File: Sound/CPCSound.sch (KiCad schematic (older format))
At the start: 8 parts, among them J903 Conn_01x08_Female

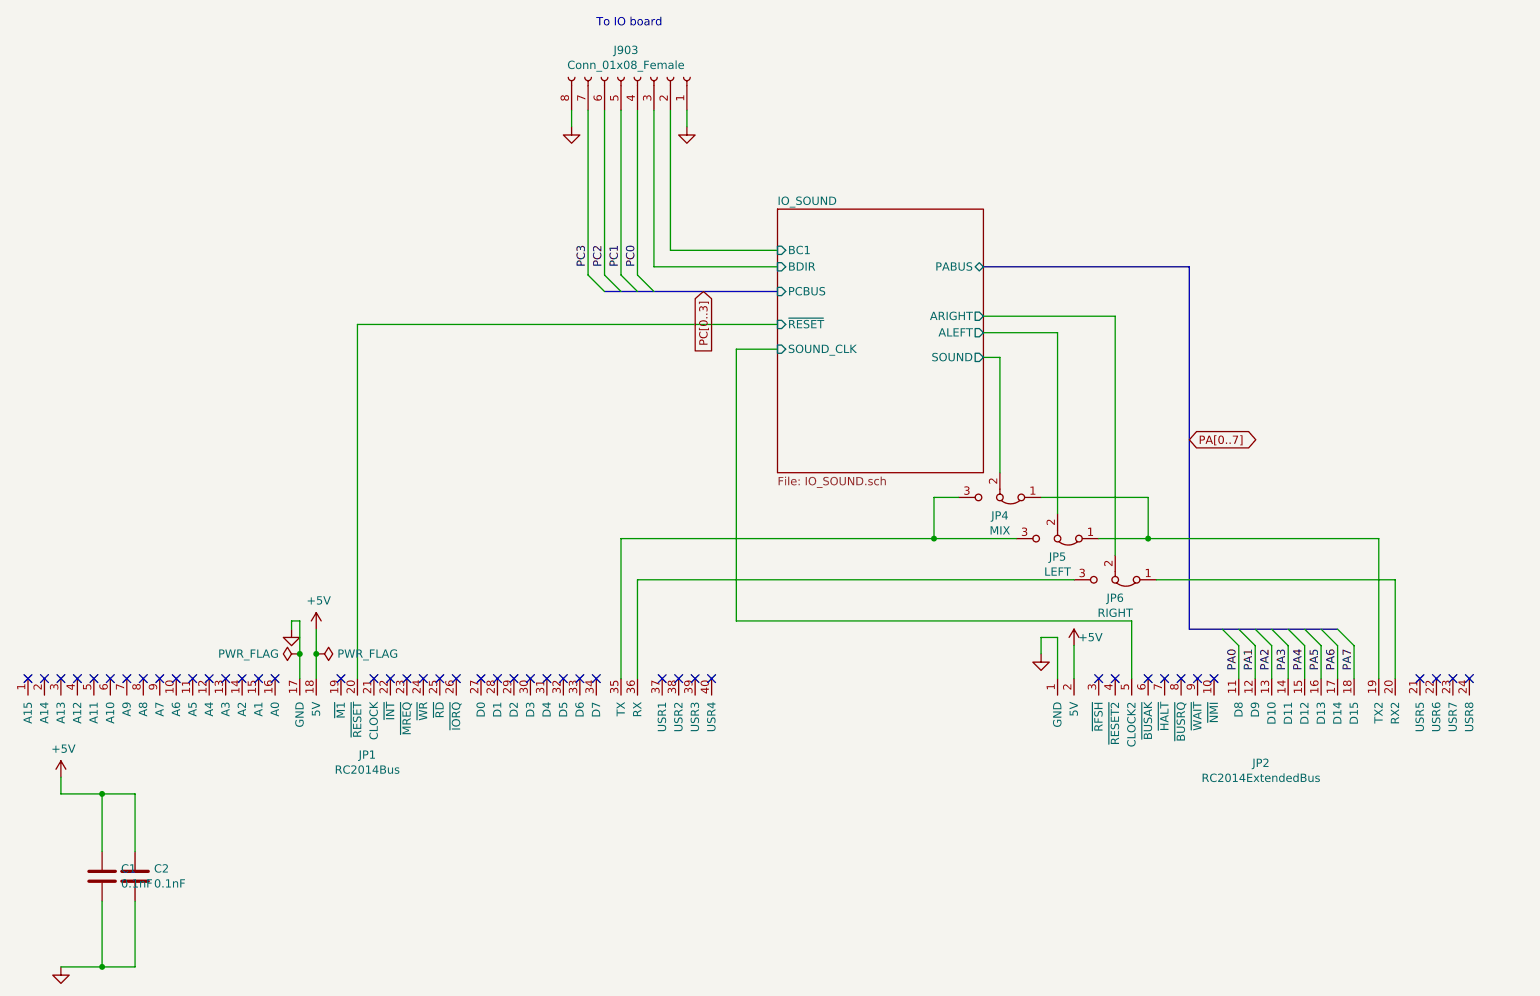
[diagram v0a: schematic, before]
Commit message: Long overdue update...
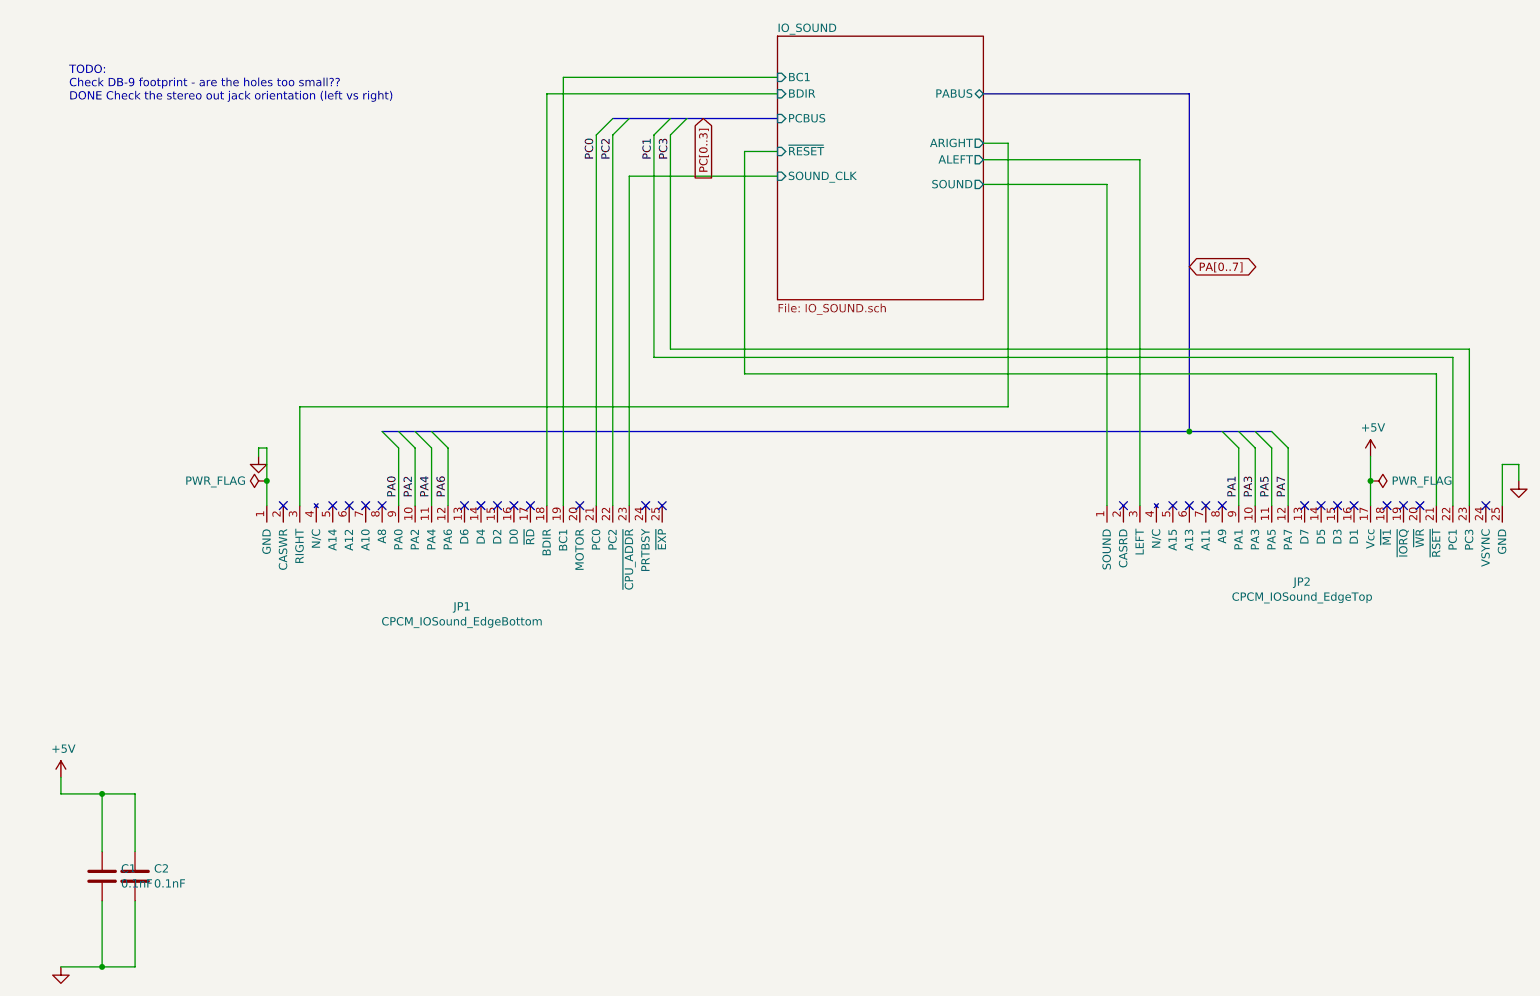
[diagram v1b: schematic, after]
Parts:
- removed J903: Conn_01x08_Female, Connector_PinSocket_2.54mm:PinSocket_1x08_P2.54mm_Vertical, symbol Connector:Conn_01x08_Female
- removed JP1: RC2014Bus, Connector_PinHeader_2.54mm:PinHeader_1x40_P2.54mm_Vertical, symbol CPCSound-rescue:RC2014Bus-CPC
- removed JP2: RC2014ExtendedBus, Connector_PinHeader_2.54mm:PinHeader_1x25_P2.54mm_Vertical, symbol CPCSound-rescue:RC2014ExtendedBus-CPC
- removed JP4: MIX, Connector_PinHeader_2.54mm:PinHeader_1x03_P2.54mm_Vertical, symbol Jumper:Jumper_3_Bridged12
- removed JP5: LEFT, Connector_PinHeader_2.54mm:PinHeader_1x03_P2.54mm_Vertical, symbol Jumper:Jumper_3_Bridged12
- removed JP6: RIGHT, Connector_PinHeader_2.54mm:PinHeader_1x03_P2.54mm_Vertical, symbol Jumper:Jumper_3_Bridged12
- added JP1: CPCM_IOSound_EdgeBottom, CPCModular:Edge25_2.54PS, symbol CPCModular:CPCM_IOSound_EdgeTop
- added JP2: CPCM_IOSound_EdgeTop, CPCModular:Edge25_2.54PS, symbol CPCModular:CPCM_IOSound_EdgeBottom
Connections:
- net +5V: now also JP2.17 (Vcc)
- net GND: now also JP1.1 (GND), JP2.25 (GND)
- net IO_SOUND/ALEFT: now also JP2.3 (LEFT)
- net IO_SOUND/ARIGHT: now also JP1.3 (RIGHT)
- net IO_SOUND/BC1: now also JP1.19 (BC1)
- net IO_SOUND/BDIR: now also JP1.18 (BDIR)
- net IO_SOUND/SOUND: now also JP2.1 (SOUND)
- net IO_SOUND/SOUND_CLK: now also JP1.23 (~CPU_ADDR)
- net IO_SOUND/~RESET: now also JP2.21 (~RSET)
- net PA0: now also JP1.9 (PA0)
- net PA1: now also JP2.9 (PA1)
- net PA2: now also JP1.10 (PA2)
- net PA3: now also JP2.10 (PA3)
- net PA4: now also JP1.11 (PA4)
- net PA5: now also JP2.11 (PA5)
- net PA6: now also JP1.12 (PA6)
- net PA7: now also JP2.12 (PA7)
- net PC0: now also JP1.21 (PC0)
- net PC1: now also JP2.22 (PC1)
- net PC2: now also JP1.22 (PC2)
- net PC3: now also JP2.23 (PC3)
- no-connect marks 46 -> 26
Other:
- note added: "TODO:\nCheck DB-9 footprint - are the holes too small??\nDONE Check the stereo out jack orientation (left vs right)"
- note removed: "To IO board"
